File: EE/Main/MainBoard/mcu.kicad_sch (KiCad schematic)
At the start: 5 parts, among them J7 TAG_CONNECT, U1 STM32C011F4U6TR

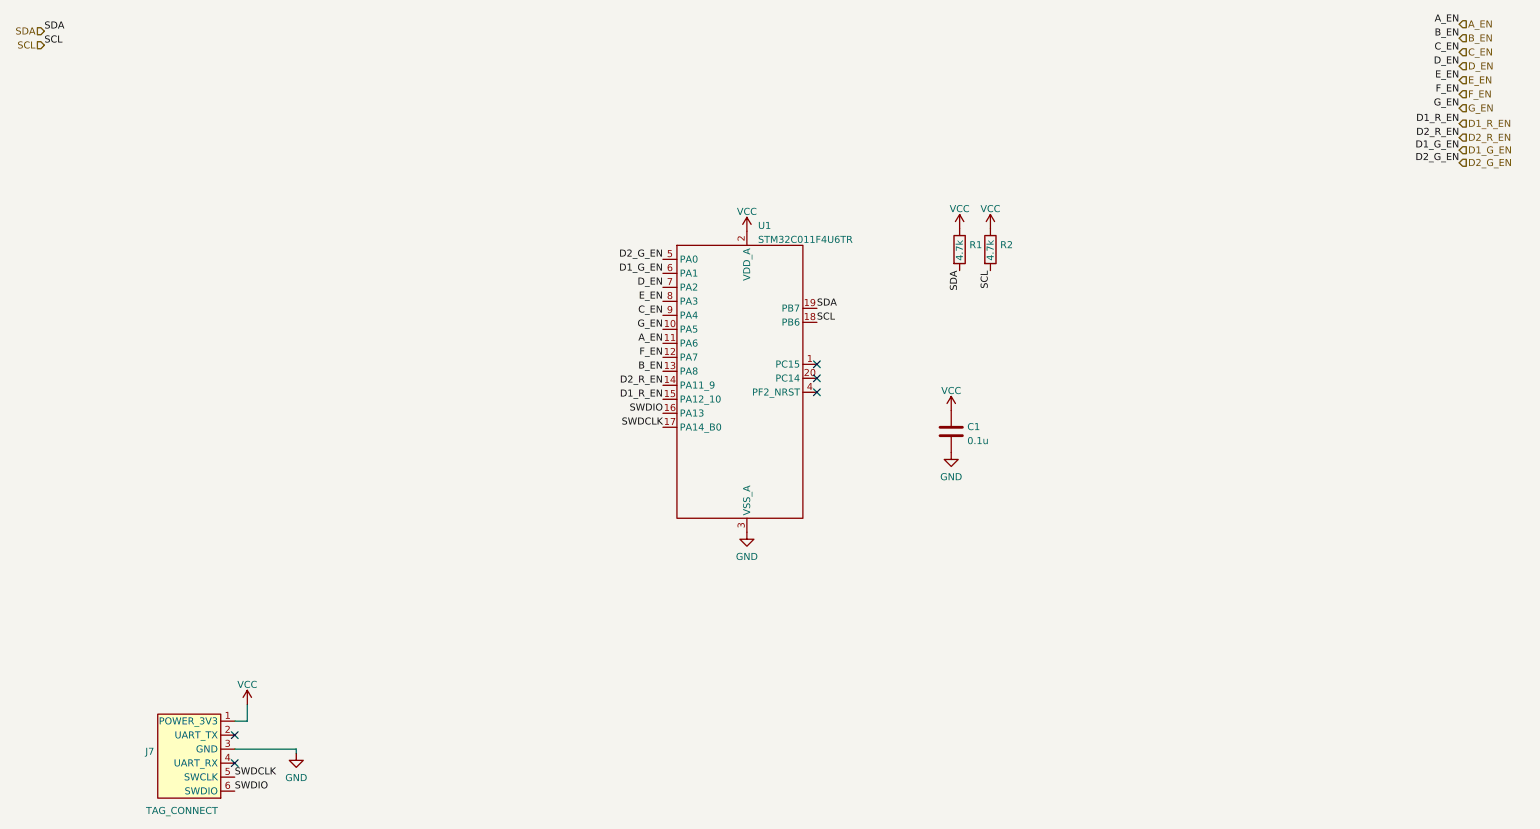
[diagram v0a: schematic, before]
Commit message: Random Check in
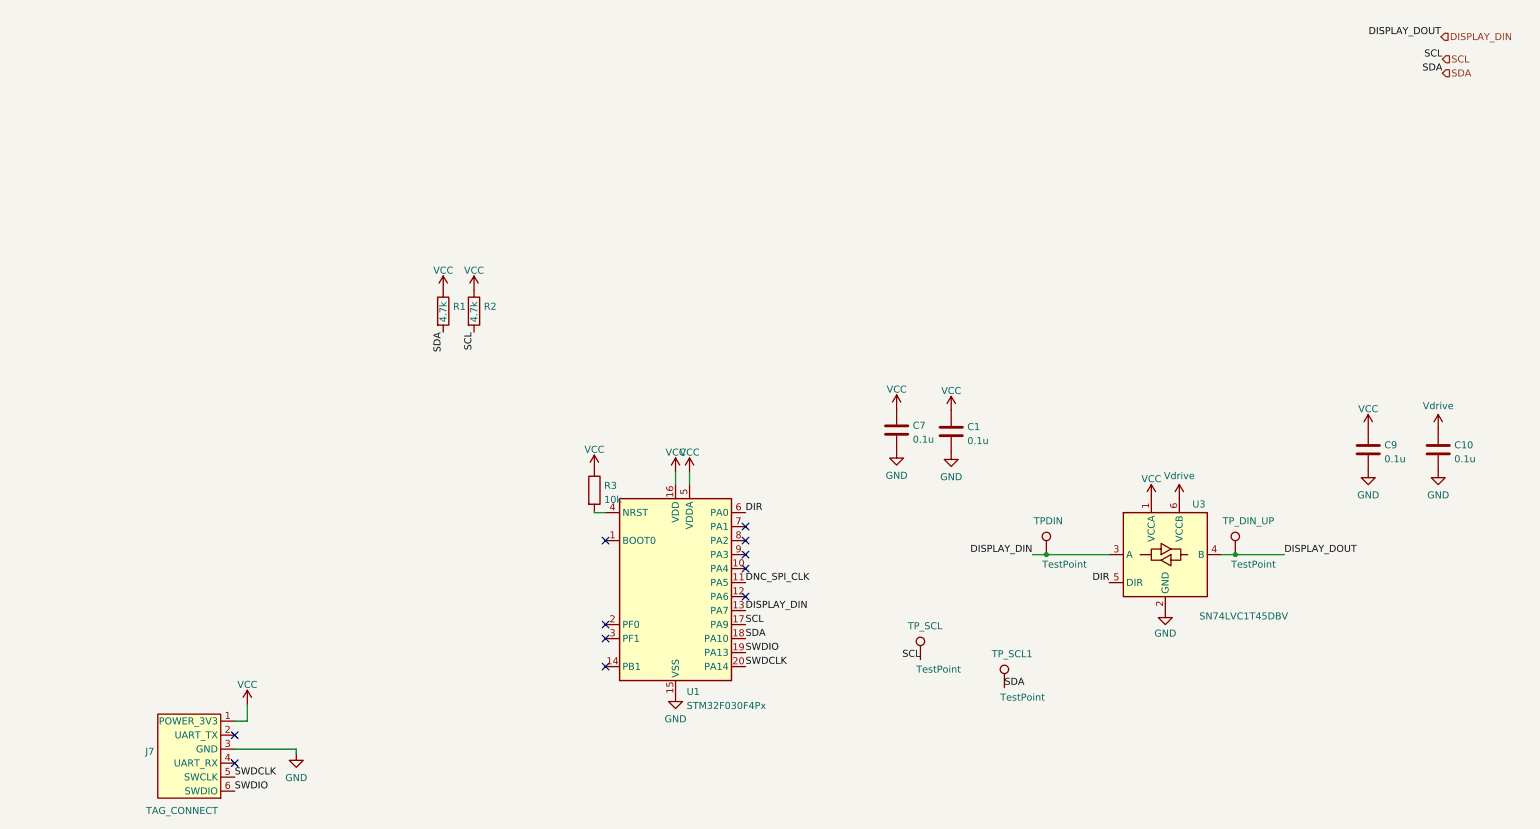
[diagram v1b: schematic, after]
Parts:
- removed U1: STM32C011F4U6TR, Package_DFN_QFN:UQFN-20_3x3mm_P0.4mm, symbol New_Library:STM32C011F4U6TR
- added C10, C7, C9: 0.1u, Capacitor_SMD:C_0402_1005Metric, symbol Device:C
- added R3: 10k, Resistor_SMD:R_0402_1005Metric, symbol Device:R
- added TPDIN, TP_DIN_UP, TP_SCL, TP_SCL1: TestPoint, TestPoint:TestPoint_Pad_1.5x1.5mm, symbol Connector:TestPoint
- added U1: STM32F030F4Px, Package_SO:TSSOP-20_4.4x6.5mm_P0.65mm, symbol MCU_ST_STM32F0:STM32F030F4Px
- added U3: SN74LVC1T45DBV, Package_TO_SOT_SMD:SOT-23-6, symbol Logic_LevelTranslator:SN74LVC1T45DBV
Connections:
- net GND: now also C10.2, C7.2, C9.2, U1.15 (VSS), U3.2 (GND)
- net SCL: now also TP_SCL.1, U1.17 (PA9)
- net SDA: now also TP_SCL1.1, U1.18 (PA10)
- net SWDCLK: now also U1.20 (PA14)
- net SWDIO: now also U1.19 (PA13)
- net VCC: now also C7.1, C9.1, R3.1, U1.16 (VDD), U1.5 (VDDA), U3.1 (VCCA)
- new net: R3.2, U1.4 (NRST)
- new net DIR: U1.6 (PA0), U3.5 (DIR)
- new net DISPLAY_DIN: TPDIN.1, TP_DIN_UP.1, U1.13 (PA7), U3.3 (A), U3.4 (B)
- new net DNC_SPI_CLK: U1.11 (PA5)
- new net Vdrive: C10.1, U3.6 (VCCB)
- no-connect marks 5 -> 11
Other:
- moved on the sheet: R1, R2
